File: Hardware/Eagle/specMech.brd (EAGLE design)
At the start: 142.2 x 121.9 mm, 77 parts, among them J1 PINHD-1X8-MOLEX-SHROUD, J3 PINHD-1X8-MOLEX-SHROUD, J4 PINHD-1X8-MOLEX-SHROUD, J6 Molex 0022232081, J8 Molex 0022232081, U1 MCP23008-E/SO, U10 ADS1115, U11 MCP23008-E/SO, U12 74HC2G17TSSOP-6, U13 ISO7421DR, U14 MB85RC256, U2 MCP23008-E/SO, U3 TXB0102DCURVSSOP8, U4 MCP9808-E/MS, U5 TBD62083, U6 DS3231MZ+, U7 LTC4311ISC6TRPBF, U8 MCP23008-E/SO, U9 ADS1115

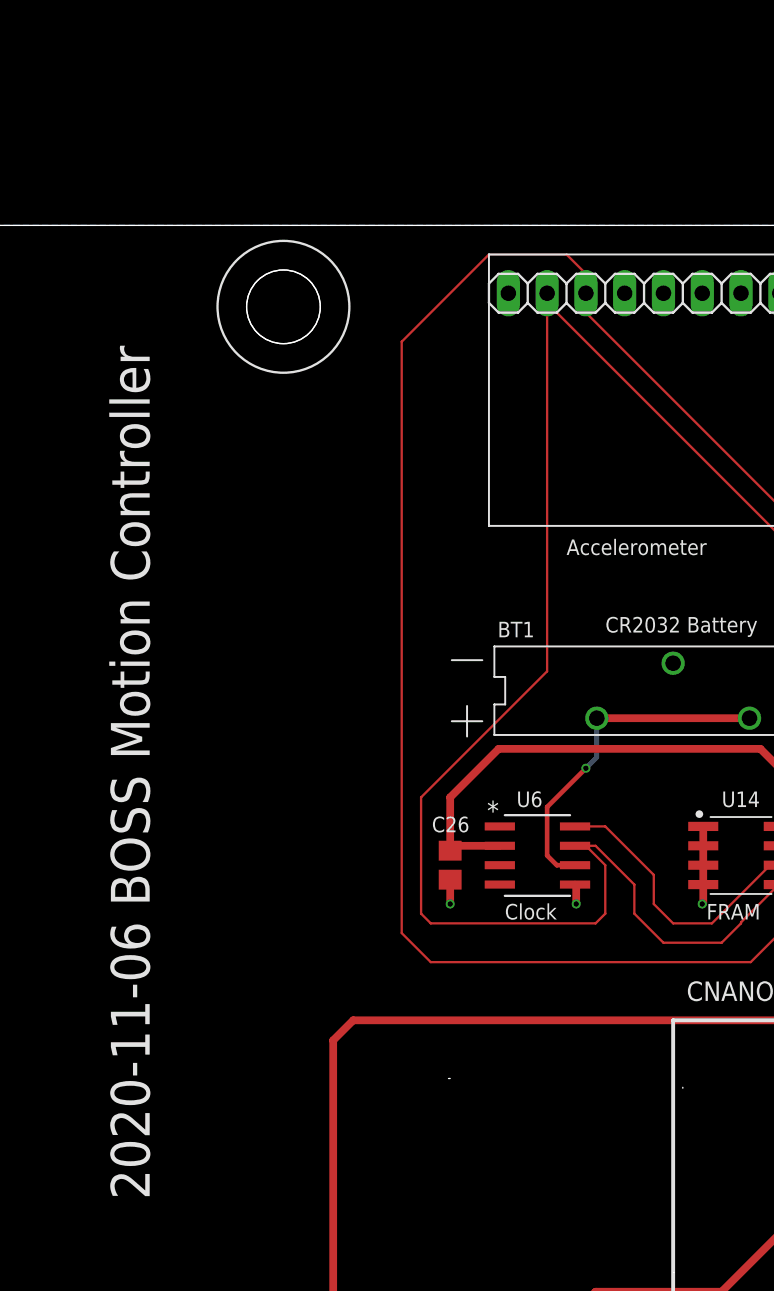
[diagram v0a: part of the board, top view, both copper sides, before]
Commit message: Connected VOFF to GND
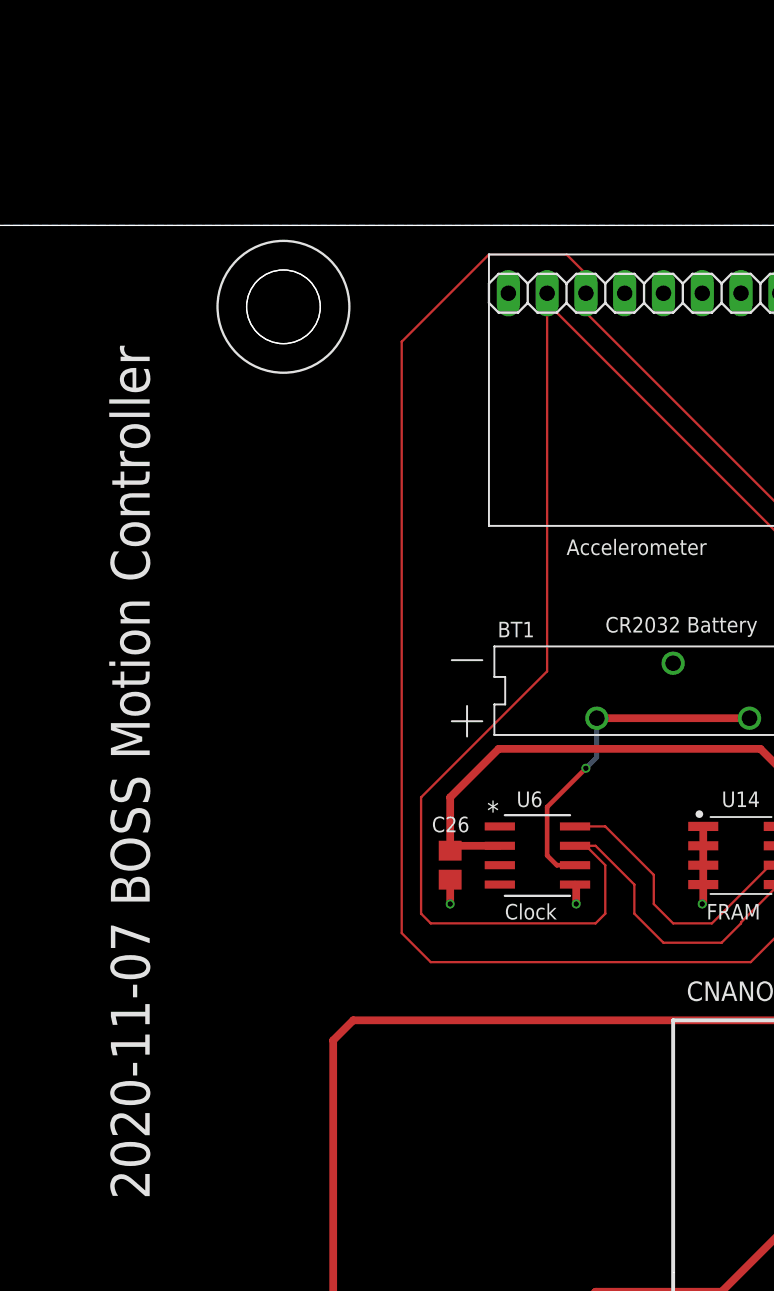
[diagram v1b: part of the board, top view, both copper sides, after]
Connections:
- net GND: now also CNANO1.VOFF
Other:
- outline, holes or cut-outs redrawn
- board text added: "2020-11-07 BOSS Motion Controller"
- board text removed: "2020-11-06 BOSS Motion Controller"
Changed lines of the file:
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@@
 <text x="127.635" y="1.905" size="1.016" layer="21" font="vector">Analog
 Corner</text>
-<text x="12.065" y="58.1025" size="2.54" layer="21" rot="R90">2020-11-06 BOSS Motion Controller</text>
+<text x="12.065" y="58.1025" size="2.54" layer="21" rot="R90">2020-11-07 BOSS Motion Controller</text>
 <wire x1="0" y1="49.53" x2="18.415" y2="49.53" width="0.254" layer="21"/>
 <wire x1="18.415" y1="49.53" x2="20.32" y2="47.625" width="0.254" layer="21"/>
@@
 <hole x="20.828" y="116.586" drill="4.826"/>
 <circle x="122.428" y="5.334" radius="2.413" width="0" layer="20"/>
-<wire x1="31.6393" y1="66.0352" x2="31.75" y2="66.04" width="0" layer="20"/>
-<wire x1="46.9876" y1="65.4603" x2="46.99" y2="65.405" width="0" layer="20"/>
 <wire x1="46.4103" y1="53.3424" x2="46.355" y2="53.34" width="0" layer="20"/>
 <circle x="20.828" y="116.586" radius="2.413" width="0" layer="20"/>
@@
 <wire x1="92.3925" y1="45.085" x2="94.2975" y2="45.085" width="0.508" layer="1"/>
 <wire x1="94.2975" y1="45.085" x2="96.52" y2="45.085" width="0.508" layer="1"/>
+<contactref element="CNANO1" pad="VOFF"/>
 </signal>
 <signal name="+5V">
